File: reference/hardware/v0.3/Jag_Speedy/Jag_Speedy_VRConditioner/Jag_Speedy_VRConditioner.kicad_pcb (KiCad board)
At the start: 2 copper layers, 35.6 x 22.9 mm, 15 parts, among them IC1 MAX9926UAEE+, J1 Conn

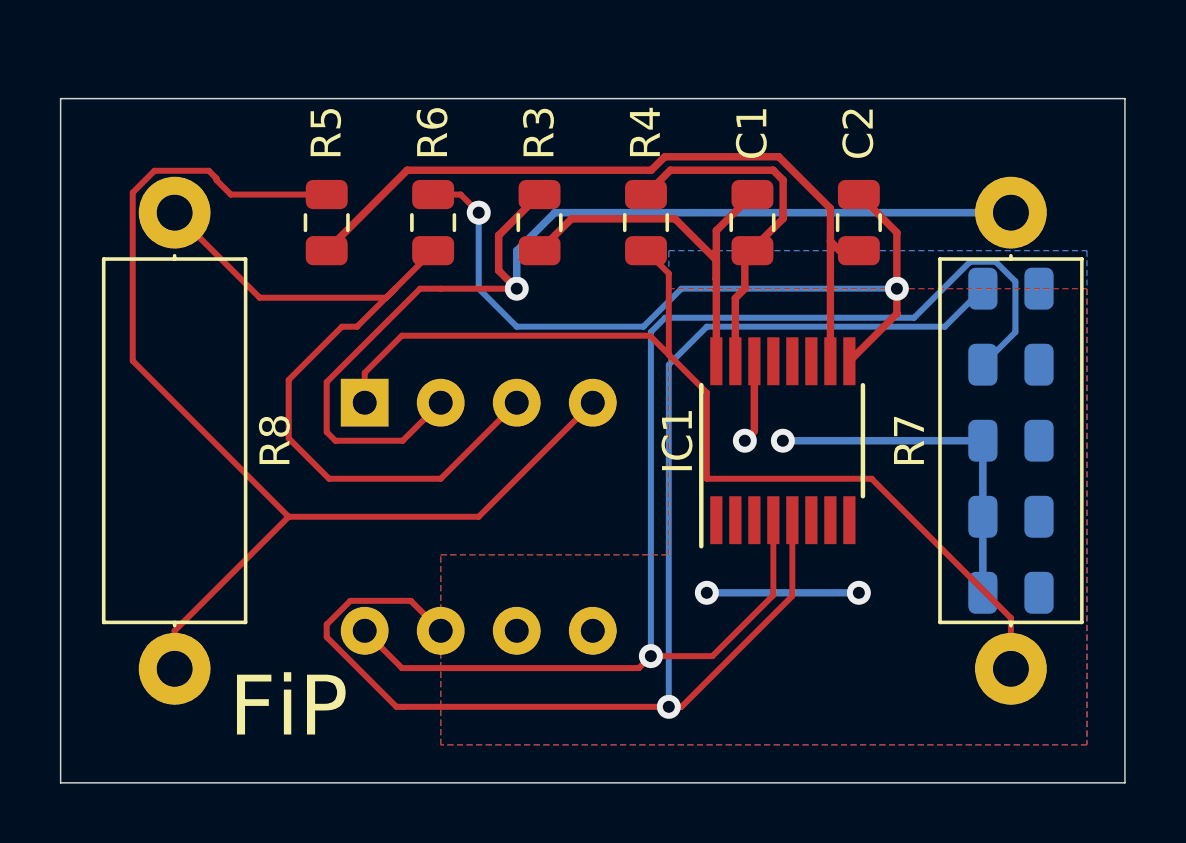
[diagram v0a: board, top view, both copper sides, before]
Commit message: PCB Changes
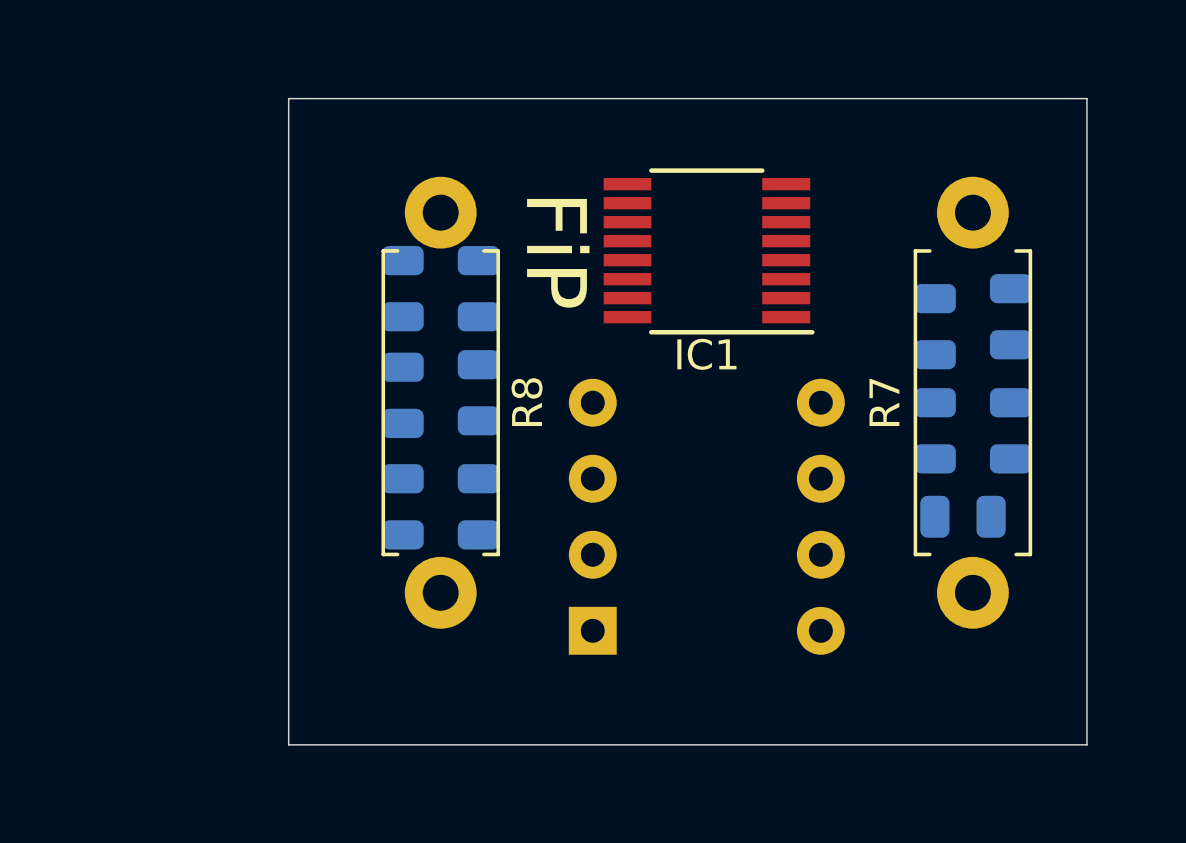
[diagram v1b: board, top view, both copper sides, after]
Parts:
- C1, C2, R3, R4, R5, R6: moved to B.Cu
- R7, R8: footprint Resistor_THT:R_Axial_DIN0414_L11.9mm_D4.5mm_P15.24mm_Horizontal -> Resistor_THT:R_Axial_DIN0411_L9.9mm_D3.6mm_P12.70mm_Horizontal
- moved C2 15.9 mm to (138.4, 92.4), turned to 270 degrees
- moved C1 15.1 mm to (135.9, 92.4), turned to 90 degrees
- moved J1 10.8 mm to (142.2, 96.5), turned to 0 degrees
- moved R8 8.89 mm to (137.2, 82.5)
- moved R4 7.97 mm to (138.4, 88.6)
- moved R3 7.36 mm to (135.9, 88.7), turned to 90 degrees
- moved IC1 6.84 mm to (146.1, 83.8), turned to 180 degrees
- moved C4 3.83 mm to (153.7, 89.8), turned to 90 degrees
- moved R5 3.37 mm to (135.9, 85.1), turned to 90 degrees
- moved C5 3.00 mm to (154.6, 92.7)
- moved R2 2.84 mm to (153.7, 86.4), turned to 270 degrees
- moved R7 2.84 mm to (154.9, 95.2)
- moved R6 2.68 mm to (138.4, 85.1)
- moved R1 1.60 mm to (156.2, 86.0), turned to 270 degrees
- moved C3 0.33 mm to (156.2, 89.8), turned to 90 degrees
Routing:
- net Output2: track 48.5 -> 0.00 mm, vias 1 -> 0
- net Output1: track 45.2 -> 0.00 mm, vias 1 -> 0
- net VR2-: track 38.5 -> 0.00 mm
- net VR1+: track 36.0 -> 0.00 mm, vias 1 -> 0
- net VR1-: track 34.2 -> 0.00 mm
- net VR2+: track 26.5 -> 0.00 mm
- net Net-(C2-Pad2): track 26.1 -> 0.00 mm, vias 2 -> 0
- net Net-(C2-Pad1): track 25.0 -> 0.00 mm
- net Ground: track 16.8 -> 0.00 mm, vias 3 -> 0
- net Net-(C1-Pad1): track 13.6 -> 0.00 mm
- net Net-(C1-Pad2): track 11.8 -> 0.00 mm
- net 5V: track 2.79 -> 0.00 mm, vias 1 -> 0
- removed copper zone on B.Cu, net 5V
- removed copper zone on F.Cu, net Ground
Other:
- board size 35.6 x 22.9 mm -> 26.7 x 21.6 mm

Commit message: PCB Rework
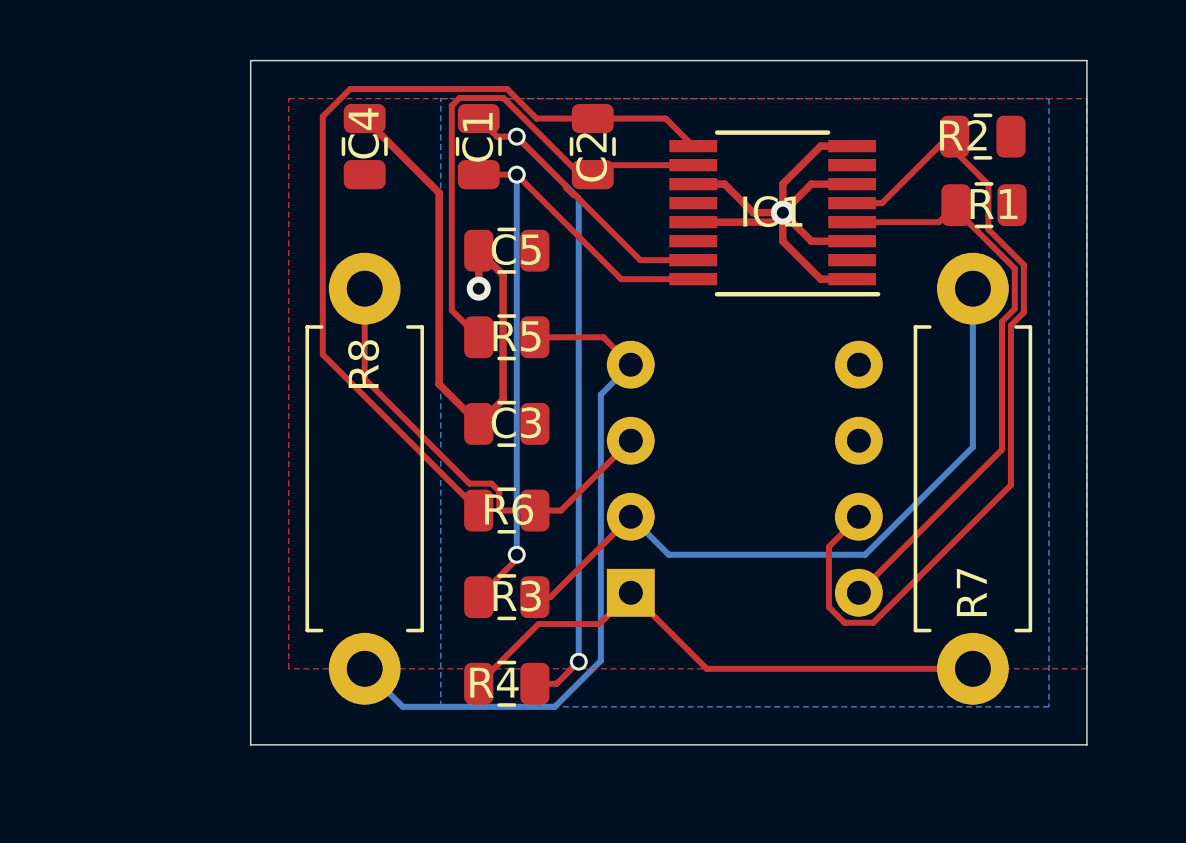
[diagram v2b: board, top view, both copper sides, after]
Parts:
- C1, C2, C3, C4, C5, R1, R2, R3, R4, R5, R6: moved to F.Cu
- moved C4 21.3 mm to (134.6, 80.3)
- moved C5 17.6 mm to (139.4, 83.8)
- moved C3 16.8 mm to (139.4, 89.6), turned to 180 degrees
- moved C2 12.6 mm to (142.2, 80.3), turned to 90 degrees
- moved C1 12.3 mm to (138.4, 80.3)
- moved R4 9.77 mm to (139.4, 98.3), turned to 0 degrees
- moved R3 7.59 mm to (139.4, 95.4), turned to 180 degrees
- moved R6 7.47 mm to (139.4, 92.5), turned to 180 degrees
- moved R2 6.55 mm to (155.3, 80.0), turned to 0 degrees
- moved R5 3.84 mm to (139.4, 86.7), turned to 180 degrees
- moved R1 3.83 mm to (155.3, 82.3), turned to 0 degrees
- moved R8 3.59 mm to (134.6, 85.1)
- moved R7 2.54 mm to (154.9, 97.8)
- moved IC1 2.54 mm to (148.2, 82.5)
- moved J1 1.80 mm to (143.5, 95.2)
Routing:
- net Ground: track 0.00 -> 39.0 mm, vias 0 -> 2
- net Net-(C1-Pad2): track 0.00 -> 29.3 mm, vias 0 -> 2
- net Net-(C2-Pad2): track 0.00 -> 28.9 mm
- net Output2: track 0.00 -> 28.8 mm
- net Net-(C1-Pad1): track 0.00 -> 23.3 mm, vias 0 -> 2
- net VR1+: track 0.00 -> 23.1 mm
- net VR2-: track 0.00 -> 22.9 mm
- net Output1: track 0.00 -> 19.6 mm
- net VR1-: track 0.00 -> 18.8 mm
- net Net-(C2-Pad1): track 0.00 -> 17.5 mm
- net VR2+: track 0.00 -> 15.1 mm
- added copper zone on F.Cu, net 5V
- added copper zone on B.Cu, net Ground
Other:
- board size 26.7 x 21.6 mm -> 27.9 x 22.9 mm
